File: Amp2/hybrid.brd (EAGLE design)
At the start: 174 x 168.9 mm, 127 parts, among them IC1 TL071P, IC2 TL071P, IC3 LM317MABT-OUT, IC4 LM317MABT-OUT, J1 RCJ-21XXMILL, J2 NRJ3HF-1, J3 703W-00/54, Q1 KSP06KINKED, Q10 BD139, Q11 KSP06KINKED, Q12 BC560KINKED, Q13 BC560KINKED, Q14 BC560KINKED, Q15 BC556KINKED, Q16 BC550KINKED, Q17 BC550KINKED, Q18 BC560KINKED, Q19 BD140, Q2 BC560KINKED, Q20 BD139, Q21 KSP43, Q3 BC560KINKED, Q4 BC560KINKED, Q5 BC556KINKED, Q6 BC550KINKED, Q7 BC550KINKED, Q8 BC560KINKED, Q9 BD140

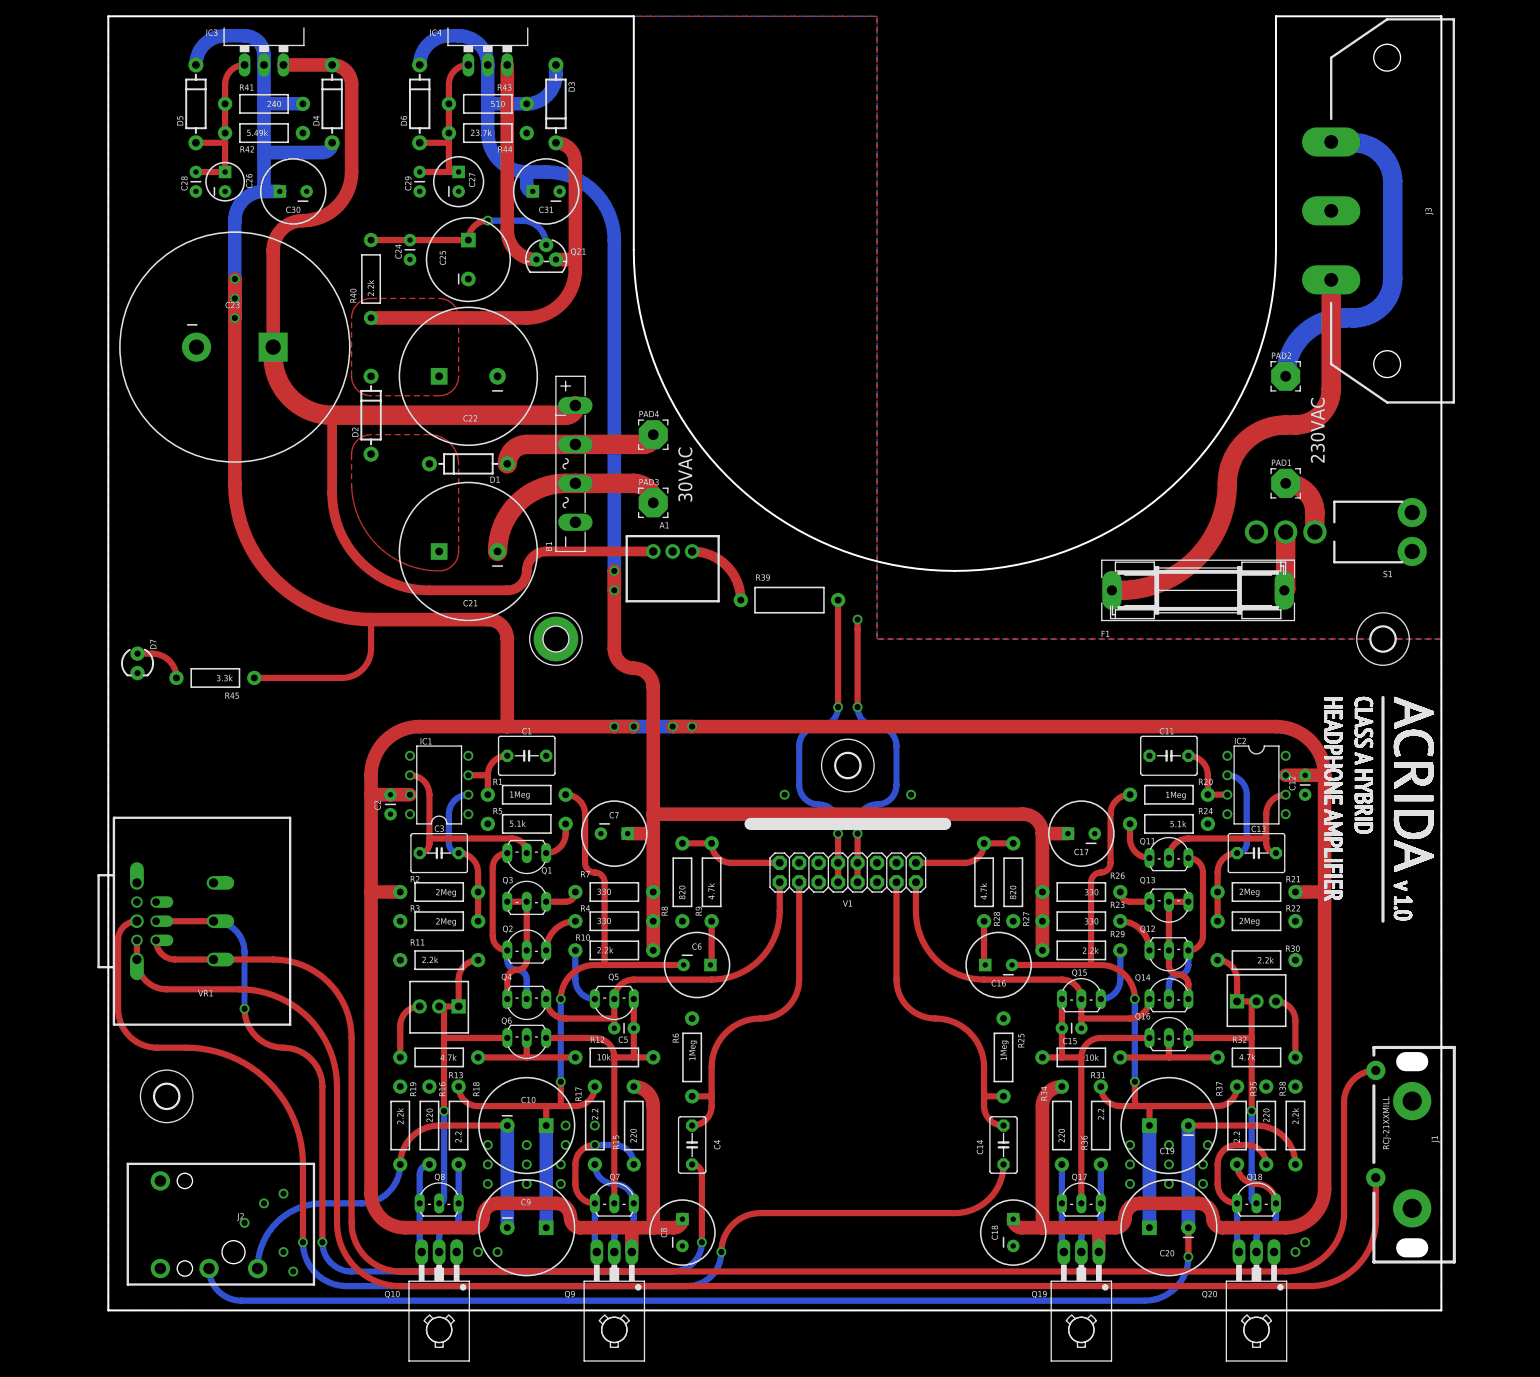
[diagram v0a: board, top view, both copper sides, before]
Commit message: New board again
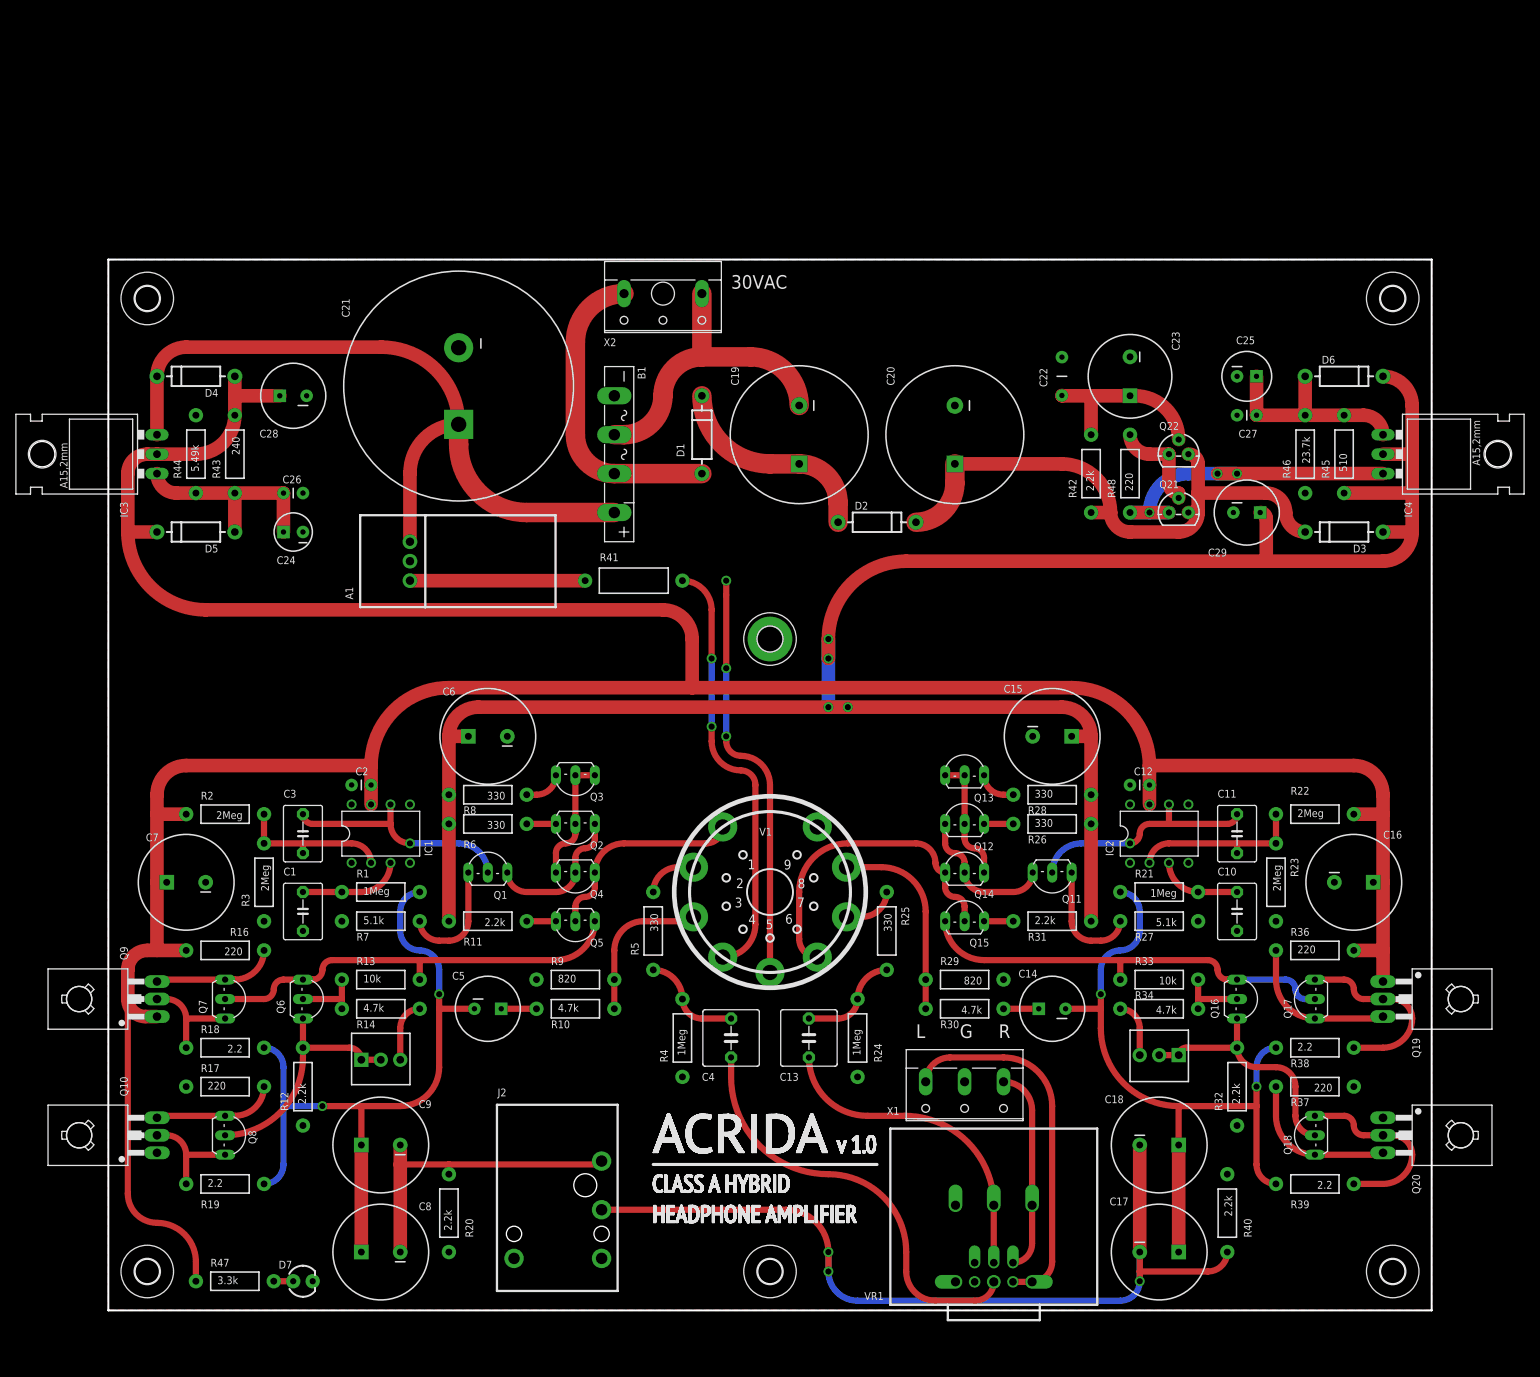
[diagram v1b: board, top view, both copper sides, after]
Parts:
- removed C30, C31: 47uF, my-cap:CPOL-RADIAL-8/3.5
- removed F1: (no value), fuse:SH22,5
- removed J1: RCJ-21XXMILL, my:RCJ-21-MILL
- removed J3: 703W-00/54, my-conn:703W-00/54
- removed PAD1, PAD2, PAD3, PAD4: (no value), wirepad:3,81/1,4
- removed S1: SW-M2012SA2W40, my-sw:SW-M2012S2A2G40
- added H5, H6: MOUNT-HOLE3.2, holes:3,2
- added Q22: KSP43, my-tran:TO-92
- added R46: 23.7k, SparkFun-Resistors:AXIAL-0.4
- added R47: 3.3k, SparkFun-Resistors:AXIAL-0.4
- added R48: 220, SparkFun-Resistors:AXIAL-0.4
- added X1: (no value), con-wago-508:W237-3E
- added X2: (no value), con-wago-508:W237-2N
- C10: value 470uF -> 1uF; device my-cap:CPOL-RADIAL-12.5/5 -> capacitor-wima:C5B5
- C12, C2: value 0.1uF -> 1uF
- C13: value 1uF -> 0.33u; device capacitor-wima:C5B5 -> capacitor-wima:C5B7.2
- C14: value 0.33u -> 100uF; device capacitor-wima:C5B3.5 -> my-cap:CPOL-RADIAL-8/3.5
- C15: value 10p -> 100uF; device SparkFun-Capacitors:CAP-PTH-SMALL -> my-cap:CPOL-RADIAL-12.5/5
- C16, C6: device my-cap:CPOL-RADIAL-8/3.5 -> my-cap:CPOL-RADIAL-12.5/5
- C17, C18, C8: value 47uF -> 470uF; device my-cap:CPOL-RADIAL-8/3.5 -> my-cap:CPOL-RADIAL-12.5/5
- C19, C20: device my-cap:CPOL-RADIAL-12.5/5 -> my-cap:CPOL-RADIAL-18/7.5
- C21: value 470uF -> 4700uF; device my-cap:CPOL-RADIAL-18/7.5 -> my-cap:CPOL-SNAPIN-30/10
- C22: value 470uF -> 1uF; device my-cap:CPOL-RADIAL-18/7.5 -> SparkFun-Capacitors:CAP-PTH-5MM
- C23: value 4700uF -> 47uF; device my-cap:CPOL-SNAPIN-30/10 -> my-cap:CPOL-RADIAL-12/5
- C24: value 1uF -> 10uF; device SparkFun-Capacitors:CAP-PTH-SMALL -> my-cap:CPOL-RADIAL-5/2.5
- C25: value 47uF -> 10uF; device my-cap:CPOL-RADIAL-12/5 -> my-cap:CPOL-RADIAL-6.5/2.5
- C26: value 10uF -> 1uF; device my-cap:CPOL-RADIAL-5/2.5 -> SparkFun-Capacitors:CAP-PTH-SMALL
- C27: value 10uF -> 1uF; device my-cap:CPOL-RADIAL-6.5/2.5 -> SparkFun-Capacitors:CAP-PTH-SMALL
- C28, C29: value 1uF -> 47uF; device SparkFun-Capacitors:CAP-PTH-SMALL -> my-cap:CPOL-RADIAL-8/3.5
- C4: device capacitor-wima:C5B3.5 -> capacitor-wima:C5B7.2
- C5: value 10p -> 100uF; device SparkFun-Capacitors:CAP-PTH-SMALL -> my-cap:CPOL-RADIAL-8/3.5
- C7: value 47uF -> 100uF; device my-cap:CPOL-RADIAL-8/3.5 -> my-cap:CPOL-RADIAL-12.5/5
- IC3, IC4: value LM317MABT-OUT -> LM317MABT; device my-reg:TO220L1-OUT -> my-reg:TO220L1
- R10, R30: value 2.2k -> 4.7k
- R12, R31: value 10k -> 2.2k
- R13: value 4.7k -> 10k
- R14: value 10k -> 4.7k; device SparkFun-Electromechanical:3362U-2 -> SparkFun-Resistors:AXIAL-0.4
- R15, R35: value 220 -> 10k; device SparkFun-Resistors:AXIAL-0.4 -> SparkFun-Electromechanical:3362U-2
- R17, R36, R37: value 2.2 -> 220
- R19, R38: value 2.2k -> 2.2
- R20: value 1Meg -> 2.2k
- R21: value 2Meg -> 1Meg
- R23: value 330 -> 2Meg
- R24: value 5.1k -> 1Meg
- R25, R6: value 1Meg -> 330
- R27: value 820 -> 5.1k
- R28: value 4.7k -> 330
- R29: value 2.2k -> 820
- R32: value 4.7k -> 2.2k
- R33: device SparkFun-Electromechanical:3362U-2 -> SparkFun-Resistors:AXIAL-0.4
- R34: value 220 -> 4.7k
- R39: value 0.51 -> 2.2; device my-res:AXIAL-0.5 -> SparkFun-Resistors:AXIAL-0.4
- R4: value 330 -> 1Meg
- R41: value 240 -> 0.51; device SparkFun-Resistors:AXIAL-0.4 -> my-res:AXIAL-0.5
- R42: value 5.49k -> 2.2k
- R43: value 510 -> 240
- R44: value 23.7k -> 5.49k
- R45: value 3.3k -> 510
- R5: value 5.1k -> 330
- R7: value 330 -> 5.1k
- R8: value 820 -> 330
- R9: value 4.7k -> 820
- V1: device my-tubes:NOVAL-HORIZONTAL -> my-tubes:NOVAL-21MM
- moved R40 165.4 mm to (146.1, 12.7), turned to 270 degrees
- moved H3 161.6 mm to (167.6, 5.08)
- moved R45 150.2 mm to (161.3, 111.8), turned to 90 degrees
- moved IC4 132.4 mm to (170.2, 111.8), turned to 270 degrees
- moved VR1 127.9 mm to (115.6, -1.27), turned to 270 degrees
- moved D6 125.8 mm to (161.3, 121.9), turned to 0 degrees
- moved D3 117.1 mm to (161.3, 101.6), turned to 180 degrees
- moved C23 116.9 mm to (133.3, 121.9), turned to 270 degrees
- moved R42 116.7 mm to (128.3, 109.2), turned to 90 degrees
- moved C29 116.7 mm to (148.6, 104.1), turned to 0 degrees
- moved H2 115.0 mm to (86.4, 5.08)
- moved H4 112.8 mm to (5.08, 5.08)
- moved LOGO1 111.3 mm to (71.1, 11.4), turned to 0 degrees
- moved R20 108.7 mm to (44.5, 12.7), turned to 90 degrees
- moved C27 108.5 mm to (149.9, 116.8), turned to 180 degrees
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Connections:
- removed net N$40: F1.1, J3.L
- removed net N$44: F1.2, S1.S
- removed net N$45: PAD1.1, S1.UP-CONNECT
- removed net P$1: J3.E
- new net N$6: R5.P$1, V1.2
- new net N$9: R25.P$1, V1.7
- net +6.3FIL: now also R41.P$2, V1.4; no longer R39.P$2, V1.7, V1.8
- net +LV: now also C21.1; no longer C23.1
- net AC_1: now also X2.2; no longer PAD4.1
- net AC_2: now also C19.2, X2.1; no longer C21.2, PAD3.1
- net CAT_L: now also R10.P$2, V1.3; no longer R8.P$2, V1.2
- net CAT_R: now also R29.P$2, R30.P$2, V1.8; no longer R27.P$2, R28.P$2, V1.16
- net FB_L: now also C5.2, C8.+, R18.P$1, R19.P$2; no longer C10.+, C6.2, R17.P$1, R18.P$2
- net FB_R: now also C14.2, C17.+, C18.+, R21.P$2, R38.P$1, R39.P$2; no longer C16.2, C19.+, C20.+, R20.P$2, R36.P$1, R37.P$2
- net FGND: now also V1.5; no longer V1.10, V1.9
- net GND: now also C10.1, C15.-, C16.-, C20.2, C21.2, C23.-, C25.2, C6.-, C7.-, R12.P$1, R17.P$1, R20.P$1, R23.P$2, R29.P$1, R32.P$1, R37.P$1, R4.P$1, R40.P$1, R46.P$2, R7.P$1, R9.P$1, X1.2; no longer C11.1, C17.2, C18.2, C23.2, C25.-, C30.2, C31.2, C7.2, C8.2, J1.1, J1.3, R11.P$1, R16.P$1, R19.P$1, R22.P$2, R25.P$1, R30.P$1, R35.P$1, R38.P$1, R42.P$2, R5.P$1, R6.P$1, R8.P$1, V1.11, V1.12, V1.14, V1.4, V1.5, V1.6
- net G_L: now also R4.P$2, R5.P$2; no longer R6.P$2, V1.3
- net G_R: now also C13.2, R24.P$2; no longer C14.2, V1.13
- net HT: now also C15.+, C29.1, C6.+, R11.P$2, R28.P$2, R31.P$2, R45.P$1, R6.P$2, R8.P$2; no longer C17.1, C31.1, C7.1, R10.P$2, R23.P$2, R29.P$2, R4.P$2, R43.P$1, R7.P$2
- net IN_L: now also VR1.1.2; no longer VR1.2.2.1, VR1.2.2.2
- net IN_L*: now also VR1.1.3.1, VR1.1.3.2, X1.3; no longer J1.4, VR1.2.3.1, VR1.2.3.2
- net IN_R: now also C13.1, VR1.2.2.1, VR1.2.2.2; no longer C14.1, VR1.1.2
- net IN_R*: now also VR1.2.3.1, VR1.2.3.2, X1.1; no longer J1.2, VR1.1.3.1, VR1.1.3.2
- net N$10: now also R14.P$2, R15.3; no longer R13.P$2, R14.3
- net N$11: now also R18.P$2; no longer R17.P$2
- net N$12: now also R12.P$2, R15.1, R15.2; no longer R11.P$2, R14.1, R14.2
- net N$13: now also R19.P$1; no longer R18.P$1
- net N$14: now also R16.P$1; no longer R15.P$1
- net N$15: now also R17.P$2; no longer R16.P$2
- net N$16: now also R28.P$1; no longer R26.P$1
- net N$18: now also Q21.2, Q22.1, R48.P$2; no longer J3.N, PAD2.1
- net N$19: now also C14.1, R30.P$1; no longer C16.1, R28.P$1
- net N$2: now also R8.P$1; no longer R7.P$1
- net N$20: now also R31.P$1; no longer R29.P$1
- net N$21: now also R33.P$2; no longer C15.2, R31.P$2
- net N$22: now also R33.P$1, R34.P$1; no longer R31.P$1, R32.P$1
- net N$23: now also R34.P$2, R35.3; no longer R32.P$2, R33.3
- net N$24: now also R32.P$2, R35.1, R35.2; no longer R30.P$2, R33.1, R33.2
- net N$25: now also R38.P$2; no longer R36.P$2
- net N$26: now also R39.P$1; no longer R37.P$1
- net N$27: now also R36.P$1; no longer R34.P$1
- net N$28: now also R37.P$2; no longer R35.P$2
- net N$3: now also R6.P$1; no longer R4.P$1
- net N$30: now also C24.1, R43.P$2, R44.P$1; no longer C28.1, R41.P$2, R42.P$1
- net N$31: now also C19.1; no longer C21.1
- net N$32: now also R41.P$1; no longer R39.P$1
- net N$33: now also C20.1, Q22.3, R42.P$1; no longer C22.1, R40.P$1
- net N$34: now also C22.1, C23.+, Q22.2, R42.P$2; no longer C24.1, C25.+, Q21.2, R40.P$2
- net N$36: now also C25.1, R45.P$2, R46.P$1; no longer C29.1, R43.P$2, R44.P$1
- net N$37: now also R48.P$1
- net N$39: now also R26.P$1; no longer R23.P$1
- net N$4: now also C5.1, R10.P$1; no longer C6.1, R9.P$1
- net N$41: now also C11.2, R23.P$1; no longer C13.2, R21.P$1
- net N$42: now also C10.2, R21.P$1; no longer C11.2, R20.P$1
- net N$43: now also C11.1; no longer C13.1
- net N$46: now also R47.P$2; no longer R45.P$2
- net N$47: now also R7.P$2; no longer R5.P$2
- net N$48: now also R27.P$2; no longer R24.P$2
- net N$5: now also R11.P$1; no longer R10.P$1
- net N$7: now also R13.P$2; no longer C5.2, R12.P$2
- net N$8: now also R14.P$1; no longer R12.P$1
- net OUT_L: now also C8.-, R20.P$2; no longer C10.-, R19.P$2
- net OUT_R: now also C17.-, C18.-, R40.P$2; no longer C19.-, C20.-, R38.P$2
- net PL_L: no longer C5.1
- net PL_R: now also V1.6; no longer C15.1, V1.15
- net VCC: now also C16.+, C28.1, C7.+, R16.P$2, R22.P$2, R36.P$2, R43.P$1, R47.P$1; no longer C18.1, C30.1, C8.1, R15.P$2, R21.P$2, R34.P$2, R41.P$1, R45.P$1
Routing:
- net IN_R*: track 201.4 -> 26.2 mm
- net IN_L*: track 212.2 -> 47.0 mm
- net VCC: track 564.7 -> 423.5 mm, vias 7 -> 0
- net IN_R: track 155.5 -> 39.9 mm, vias 2 -> 0
- net IN_L: track 118.7 -> 51.4 mm, vias 3 -> 0
- net +LV: track 152.3 -> 97.3 mm
- net N$40: track 53.8 -> 0.00 mm
- net HT: track 228.9 -> 281.4 mm, vias 2 -> 4
- net OUT_R: track 165.2 -> 114.3 mm, vias 1 -> 3
- net N$18: track 42.1 -> 12.4 mm
- net G_R: track 40.1 -> 12.8 mm
- net G_L: track 40.1 -> 12.8 mm
- net N$31: track 0.00 -> 26.1 mm
- net N$33: track 49.4 -> 74.2 mm
- net AC_1: track 20.6 -> 39.7 mm
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- removed copper zone on layer 1, net N$31
- removed copper zone on layer 1, net N$33
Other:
- board size 174 x 168.9 mm -> 172.7 x 137.2 mm
- board text added: "G"
- board text added: "L"
- board text added: "R"
- board text removed: "230VAC"
